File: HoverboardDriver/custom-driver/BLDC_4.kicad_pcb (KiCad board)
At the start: 4 copper layers, 38.5 x 65 mm, 127 parts, among them K1 SERVO, P1 HALL/Encoder, P101 CANBUS, P2 SWD, P3 PWR_COMM, P4 IN+, P5 IN-, P6 MOTOR1, P7 MOTOR2, P9 MOTOR3, Q1 IRFS7530, Q2 IRFS7530, Q3 IRFS7530, Q4 IRFS7530, Q5 IRFS7530, Q6 IRFS7530, U1 STM32F40X_LQFP64, U2 TC2117, U3 DRV8302, U401 SN65HVD232, X1 MINI-USB-SHIELD-32005-201, X2 8MHz 10ppm

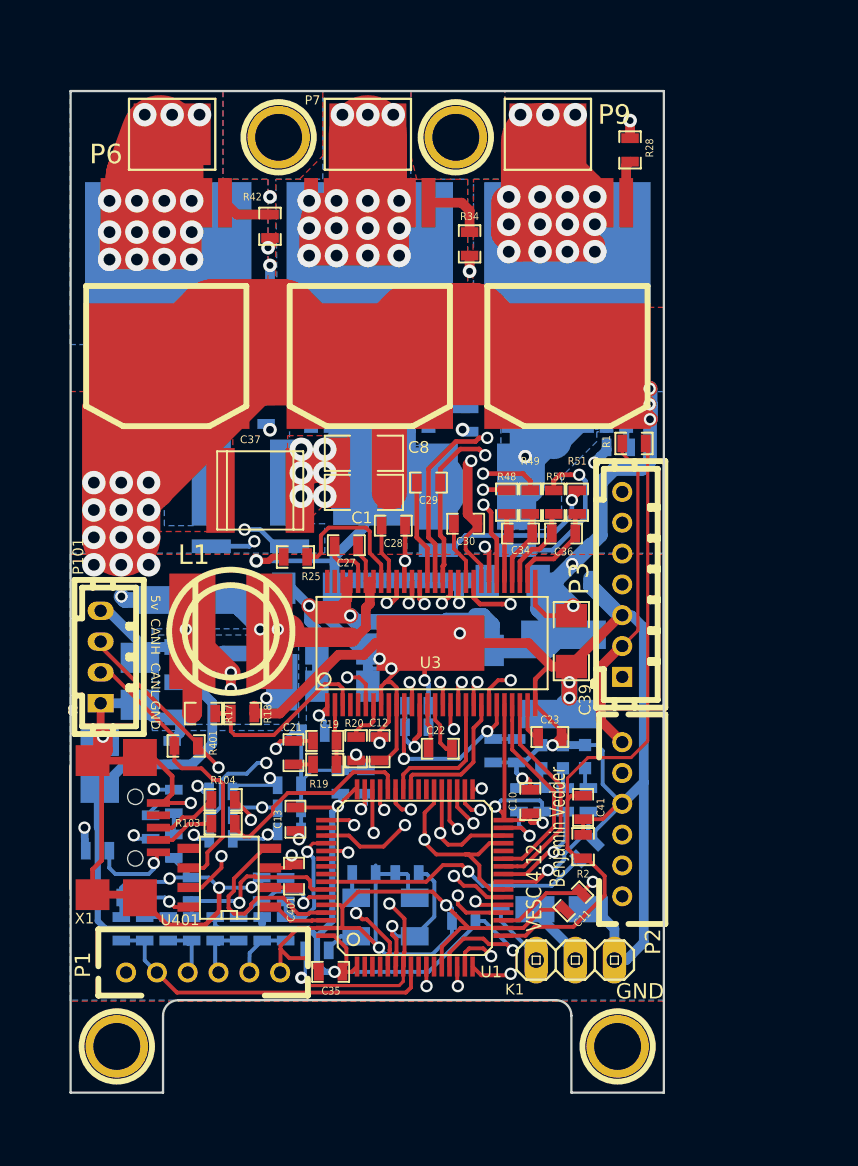
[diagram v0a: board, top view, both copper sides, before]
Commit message: New Project, SnapEDA Footprints.
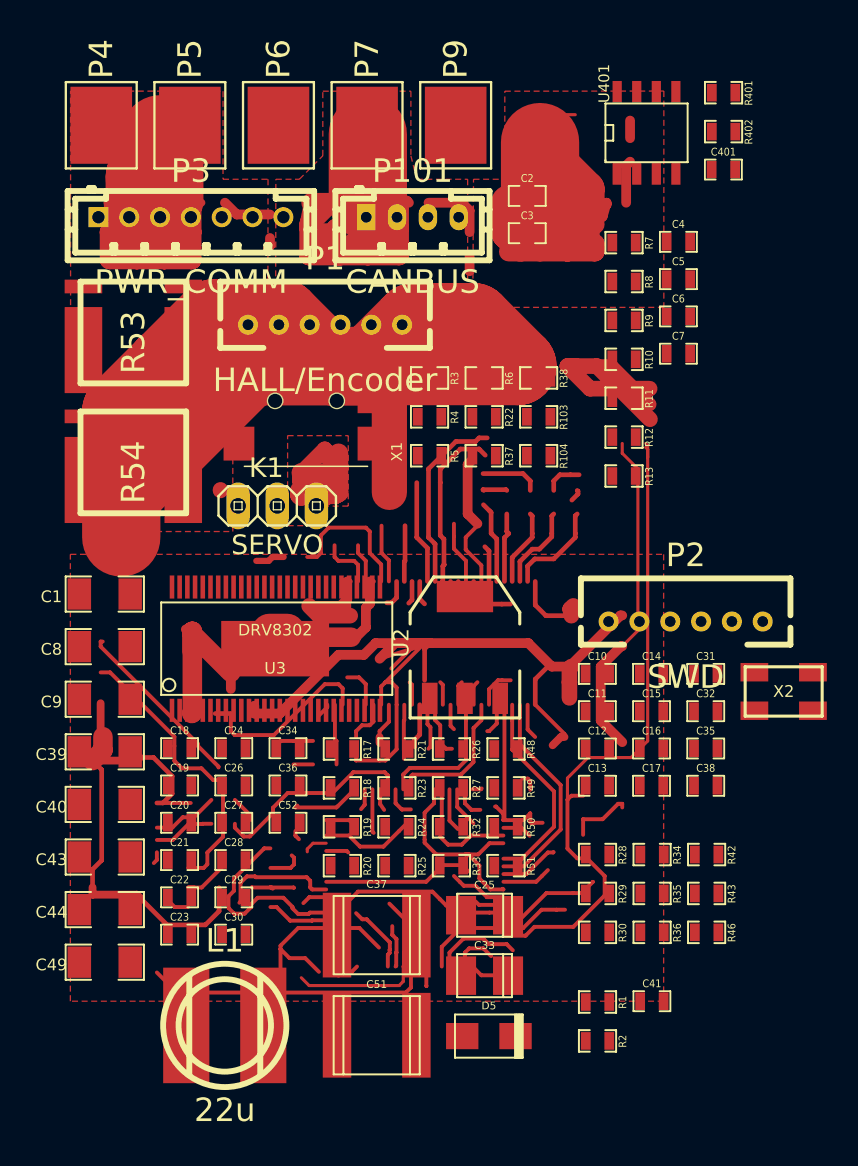
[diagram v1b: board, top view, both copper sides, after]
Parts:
- removed 1PIN (x2): P***, 1pin
- removed 1PIN (x2): P***, Connect:1pin
- removed D1: GREEN, LEDs:LED-0603
- removed D2: RED, LEDs:LED-0603
- removed D3: LED, LEDs:LED-0603
- removed D4: DIODESCH, Diodes_SMD:SMA_Handsoldering
- removed G***: oshw_silkscreen-back_3mm, oshw_silkscreen-back_3mm
- removed Q1, Q2, Q3, Q4, Q5, Q6: IRFS7530, CRF1:D2PAK-7-GDS
- removed U1: STM32F40X_LQFP64, CRF1:lqfp64_pad_mod
- C14, C15, C16, C17, C18, C2, C20, C24, C25, C26, C3, C31, C32, C33, C38, C4, C40, C43, C44, C49, C5, C51, C52, C6, C7, C9, D5, P4, P5, R10, R11, R12, R13, R21, R22, R23, R24, R26, R27, R29, R3, R30, R32, R33, R35, R36, R37, R38, R4, R402, R43, R46, R5, R53, R54, R6, R7, R8, R9, U2, X2: moved to F.Cu
- moved R402 62.8 mm to (120.9, 82.6), turned to 0 degrees
- moved C4 57.4 mm to (117.9, 89.8), turned to 0 degrees
- moved U401 55.4 mm to (115.9, 82.7), turned to 0 degrees
- moved R401 54.9 mm to (120.9, 80.1), turned to 0 degrees
- moved R7 54.3 mm to (114.4, 89.8), turned to 0 degrees
- moved C401 53.7 mm to (120.9, 85.1), turned to 0 degrees
- moved R8 50.5 mm to (114.4, 92.4), turned to 0 degrees
- moved R42 49.7 mm to (119.8, 129.5), turned to 0 degrees
- moved C2 47.7 mm to (108.1, 86.8), turned to 0 degrees
- moved C5 47.1 mm to (117.9, 92.2), turned to 0 degrees
- moved C7 47.0 mm to (117.9, 97.0), turned to 0 degrees
- moved R9 46.7 mm to (114.4, 94.9), turned to 0 degrees
- moved R46 46.4 mm to (119.8, 134.6), turned to 0 degrees
- moved C6 46.0 mm to (117.9, 94.6), turned to 0 degrees
- moved R28 45.8 mm to (112.7, 129.5), turned to 0 degrees
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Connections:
- net /Filters/TEMP_IN renamed /Filters/TEMP_MOTOR
- C16 pad 1: Net-(C16-Pad1) -> unconnected-(C16-Pad1)
- C17 pad 1: Net-(C17-Pad1) -> unconnected-(C17-Pad1)
- P2 pad 6: Net-(P2-Pad6) -> unconnected-(P2-Pad6)
- P3 pad 4: /MCU/SCK_ADC_EXT -> /SCK_ADC_EXT
- P3 pad 5: /MCU/TX_SDA_NSS -> /TX_SDA
- P3 pad 6: /MCU/RX_SCL_MOSI -> /RX_SCL_MOSI
- P3 pad 7: /MCU/MISO_ADC_EXT2 -> /MISO_RX_SCL
- R28 pad 1: Net-(Q1-PadG) -> unconnected-(R28-Pad1)
- R34 pad 1: Net-(Q3-PadG) -> unconnected-(R34-Pad1)
- R42 pad 1: Net-(Q5-PadG) -> unconnected-(R42-Pad1)
- U3 pad 4: Net-(U3-Pad4) -> unconnected-(U3-PWRGD-Pad4)
- U3 pad 5: Net-(U3-Pad5) -> unconnected-(U3-OCTW-Pad5)
- U3 pad 55: Net-(U3-Pad55) -> unconnected-(U3-EN_BUCK-Pad55)
- U3 pad 56: Net-(U3-Pad56) -> unconnected-(U3-SS_TR-Pad56)
- U401 pad 5: Net-(U401-Pad5) -> unconnected-(U401-Vref-Pad5)
- X1 pad 4: Net-(X1-Pad4) -> unconnected-(X1-Pad4)
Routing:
- net GND: track 398.8 -> 194.9 mm, vias 27 -> 0
- net VCC: track 185.2 -> 100.3 mm, vias 9 -> 0
- net V_SUPPLY: track 290.3 -> 236.8 mm, vias 20 -> 0
- net /MCU/TX_SDA_NSS: track 47.1 -> 0.00 mm, vias 2 -> 0
- net /TX_SDA: track 0.00 -> 46.8 mm
- net /RX_SCL_MOSI: track 0.00 -> 41.6 mm
- net /MCU/RX_SCL_MOSI: track 41.6 -> 0.00 mm, vias 1 -> 0
- net /MISO_RX_SCL: track 0.00 -> 36.0 mm
- net /MCU/MISO_ADC_EXT2: track 36.0 -> 0.00 mm, vias 1 -> 0
- net /Mosfet driver/H2_VS: track 145.0 -> 116.7 mm, vias 17 -> 0
- net /Mosfet driver/H1_LOW: track 48.5 -> 21.7 mm, vias 2 -> 0
- net /SCK_ADC_EXT: track 0.00 -> 26.4 mm
- net /MCU/SCK_ADC_EXT: track 26.4 -> 0.00 mm, vias 1 -> 0
- net /Mosfet driver/H3_LOW: track 53.5 -> 29.8 mm, vias 2 -> 0
- net /Mosfet driver/H3_VS: track 166.9 -> 145.9 mm, vias 18 -> 0
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- added copper zone on In1.Cu, net /Mosfet driver/H1_VS
- added copper zone on In2.Cu, net /Mosfet driver/H1_VS
- added copper zone on In1.Cu, net /Mosfet driver/H2_VS
- added copper zone on In2.Cu, net /Mosfet driver/H2_VS
- added copper zone on In1.Cu, net /Mosfet driver/H3_VS
- added copper zone on In2.Cu, net /Mosfet driver/H3_VS
- added copper zone on In1.Cu, net GND
- added copper zone on In2.Cu, net GND
- removed copper zone on B.Cu, net /Mosfet driver/H1_LOW
- removed copper zone on B.Cu, net /Mosfet driver/H1_VS
- removed copper zone on GND, net /Mosfet driver/H1_VS
- removed copper zone on GND2, net /Mosfet driver/H1_VS
- removed copper zone on B.Cu, net /Mosfet driver/H2_VS
- removed copper zone on GND, net /Mosfet driver/H2_VS
- removed copper zone on GND2, net /Mosfet driver/H2_VS
- removed copper zone on B.Cu, net /Mosfet driver/H3_LOW
- removed copper zone on B.Cu, net /Mosfet driver/H3_VS
- removed copper zone on GND, net /Mosfet driver/H3_VS
- removed copper zone on GND2, net /Mosfet driver/H3_VS
- removed copper zone on B.Cu, net GND
- removed copper zone on GND, net GND
- removed copper zone on GND2, net GND
- removed copper zone on B.Cu, net VCC
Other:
- board outline removed
- net class Default removed
- board text removed: "3.3V"
- board text removed: "3.3v"
- board text removed: "5v"
- board text removed: "ADC"
- board text removed: "ADC2"
- board text removed: "Benjamin Vedder"
- board text removed: "CANH"
- board text removed: "CANL"
- board text removed: "CLK"
- board text removed: "DIO"
- board text removed: "GND"
- board text removed: "H1"
- board text removed: "H2"
- board text removed: "H3"
- board text removed: "MISO"
- board text removed: "MOSI"
- board text removed: "NSS"
- board text removed: "RST"
- board text removed: "RX"
- board text removed: "SCK"
- board text removed: "SCL"
- board text removed: "SDA"
- board text removed: "TEMP"
- board text removed: "TX"
- board text removed: "VESC 4.12"
- board text removed: "vedder.se"
